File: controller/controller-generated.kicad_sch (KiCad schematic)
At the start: 12 parts, among them J1 USB-C, J2 Thermocouple, J3 IEC C14, J4 Cooktop, SW1 Rotary Encoder, U1 ESP32-DevKitC, U2 MAX31856

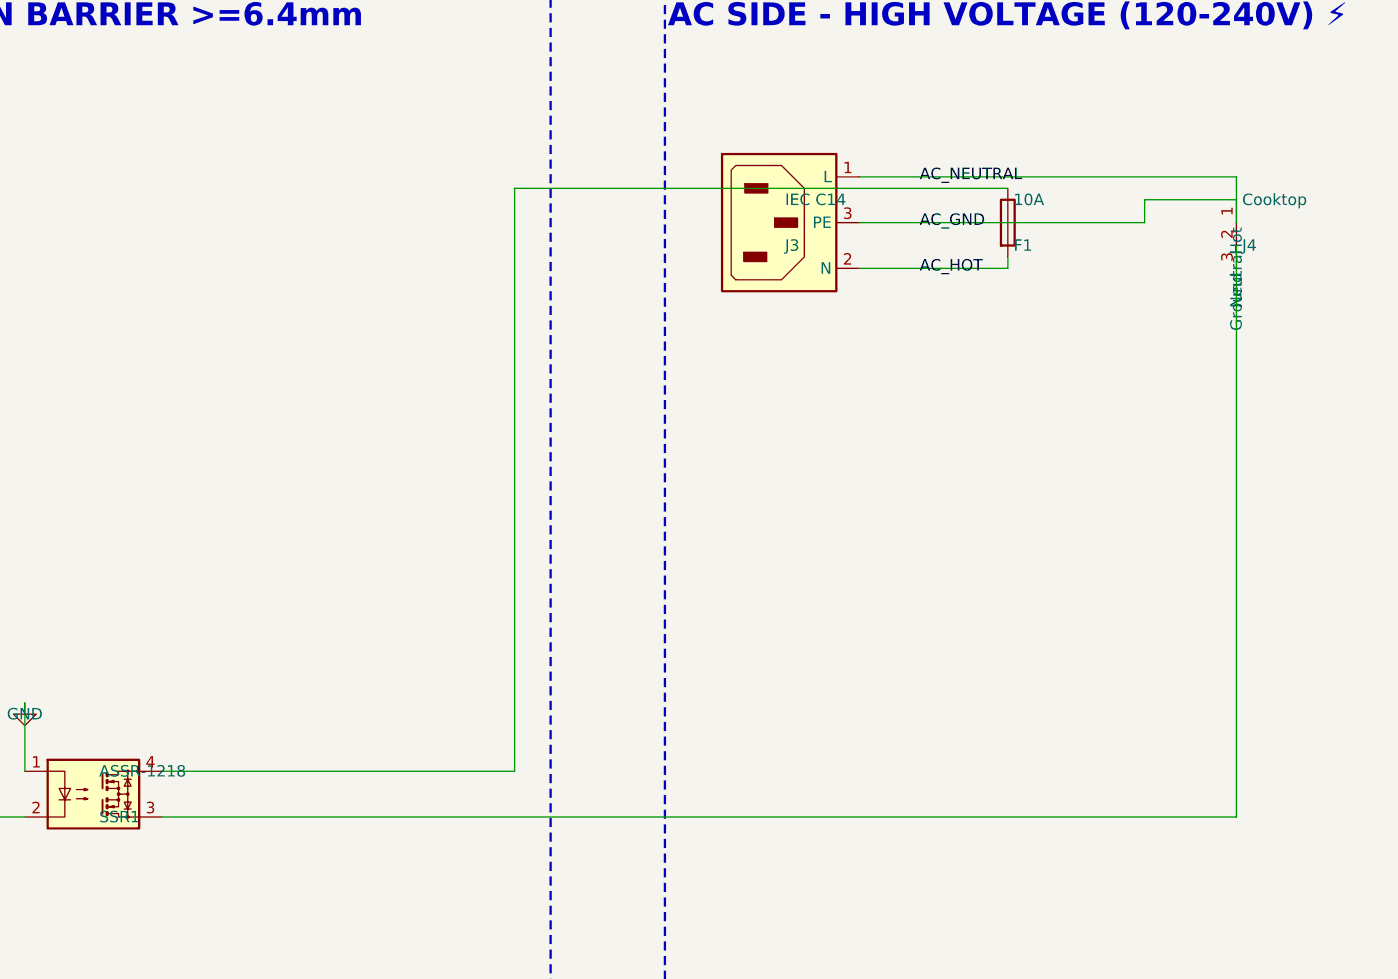
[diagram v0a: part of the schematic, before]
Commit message: fix: stabilize ac net connections
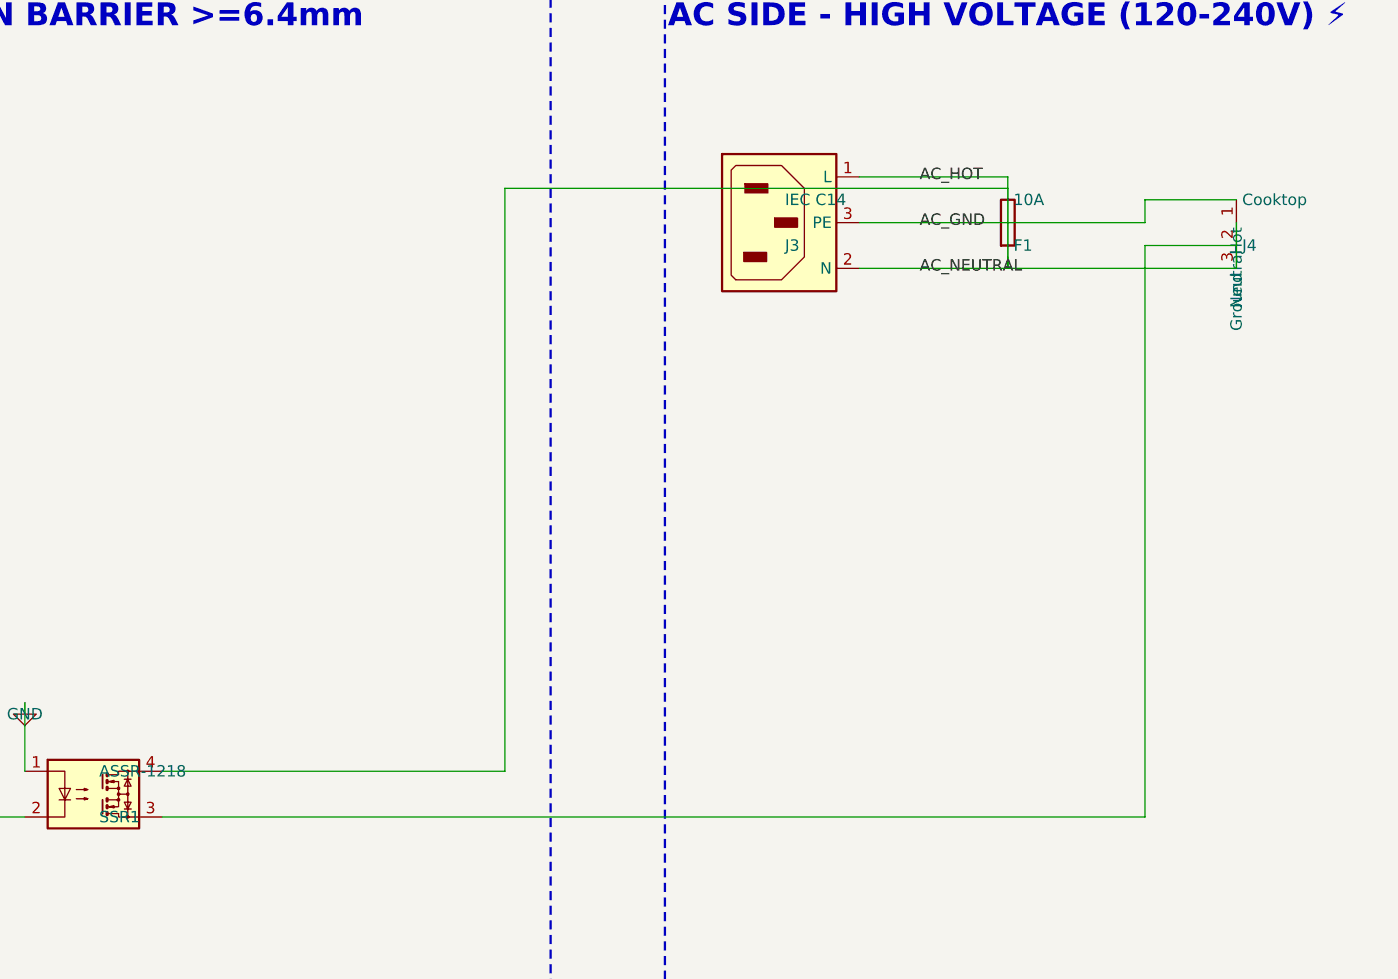
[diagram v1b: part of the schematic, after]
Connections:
- net AC_HOT: now also J3.1 (L); no longer J3.2 (N)
- net AC_NEUTRAL: now also J3.2 (N); no longer J3.1 (L)
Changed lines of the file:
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@@
 (wire
   (pts
-    (xy 288.29 68.58) (xy 304.8 68.58)
+    (xy 288.29 58.42) (xy 304.8 58.42)
+  )
+  (stroke
+    (width 0.2032)
+    (type default)
+  )
+)
+(wire
+  (pts
+    (xy 304.8 58.42) (xy 304.8 68.58)
   )
   (stroke
@@
 (wire
   (pts
-    (xy 304.8 59.69) (xy 250.0 59.69)
+    (xy 304.8 59.69) (xy 248.92 59.69)
   )
   (stroke
@@
 (wire
   (pts
-    (xy 250.0 59.69) (xy 250.0 124.46)
+    (xy 248.92 59.69) (xy 248.92 124.46)
   )
   (stroke
@@
 (wire
   (pts
-    (xy 250.0 124.46) (xy 210.82 124.46)
+    (xy 248.92 124.46) (xy 210.82 124.46)
   )
   (stroke
@@
 (wire
   (pts
-    (xy 210.82 129.54) (xy 330.2 129.54)
+    (xy 210.82 129.54) (xy 320.04 129.54)
   )
   (stroke
@@
 (wire
   (pts
-    (xy 330.2 129.54) (xy 330.2 66.04)
+    (xy 320.04 129.54) (xy 320.04 66.04)
   )
   (stroke
@@
 (wire
   (pts
-    (xy 288.29 58.42) (xy 330.2 58.42)
+    (xy 320.04 66.04) (xy 330.2 66.04)
   )
   (stroke
@@
 (wire
   (pts
-    (xy 330.2 58.42) (xy 330.2 63.5)
+    (xy 288.29 68.58) (xy 330.2 68.58)
   )
   (stroke
@@
 (wire
   (pts
-    (xy 288.29 63.5) (xy 320.0 63.5)
+    (xy 330.2 68.58) (xy 330.2 63.5)
   )
   (stroke
@@
 (wire
   (pts
-    (xy 320.0 63.5) (xy 320.0 60.96)
+    (xy 288.29 63.5) (xy 320.04 63.5)
   )
   (stroke
@@
 (wire
   (pts
-    (xy 320.0 60.96) (xy 330.2 60.96)
+    (xy 320.04 63.5) (xy 320.04 60.96)
+  )
+  (stroke
+    (width 0.2032)
+    (type default)
+  )
+)
+(wire
+  (pts
+    (xy 320.04 60.96) (xy 330.2 60.96)
   )
   (stroke
@@
   (effects (font (size 1.27 1.27)) (justify left))
 )
-(label "AC_HOT" (at 295.0 68.58 0)
+(label "AC_HOT" (at 295.0 58.42 0)
   (effects (font (size 1.27 1.27)) (justify left))
 )
-(label "AC_NEUTRAL" (at 295.0 58.42 0)
+(label "AC_NEUTRAL" (at 295.0 68.58 0)
   (effects (font (size 1.27 1.27)) (justify left))
 )
